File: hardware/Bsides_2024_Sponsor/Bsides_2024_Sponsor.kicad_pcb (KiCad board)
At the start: 2 copper layers, 139.6 x 139.6 mm, 43 parts, among them J2 Battery, J3 Battery, J4 OLED, J5 Add_On, P1 USB_C_Plug_USB2.0, Q1 DMG3415U-7, SW1 ON, SW2 RESET, SW3 BOOT, SW4 RESET, SW6 RESET, U1 ESP32-C6-WROOM-1U-N4, U2 AP2112K-3.3

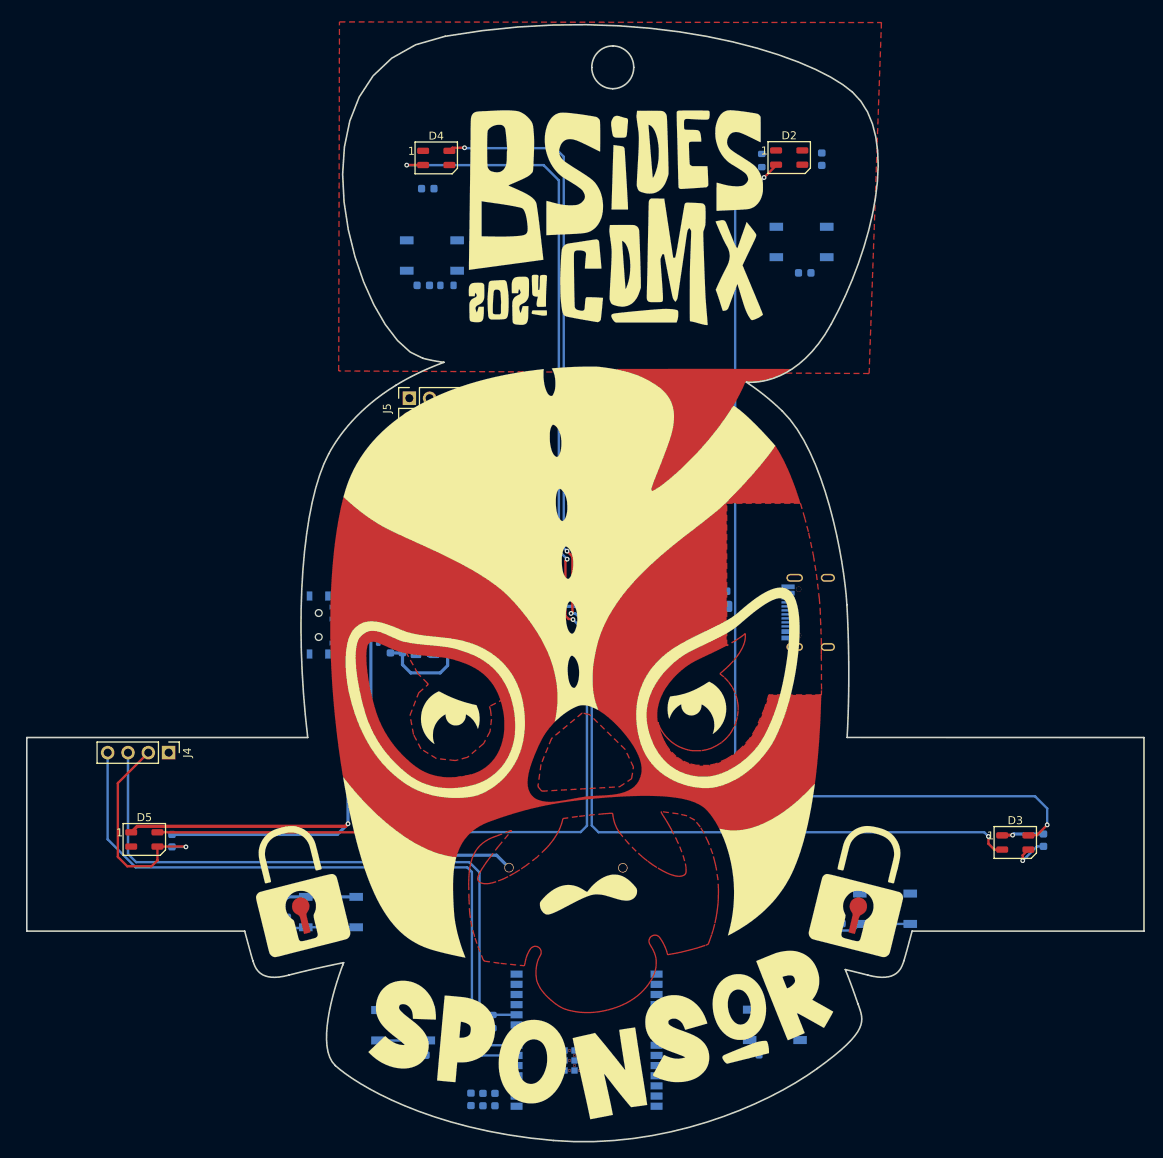
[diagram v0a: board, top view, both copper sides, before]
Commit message: feat(Hw):Update_Route_Sponsor
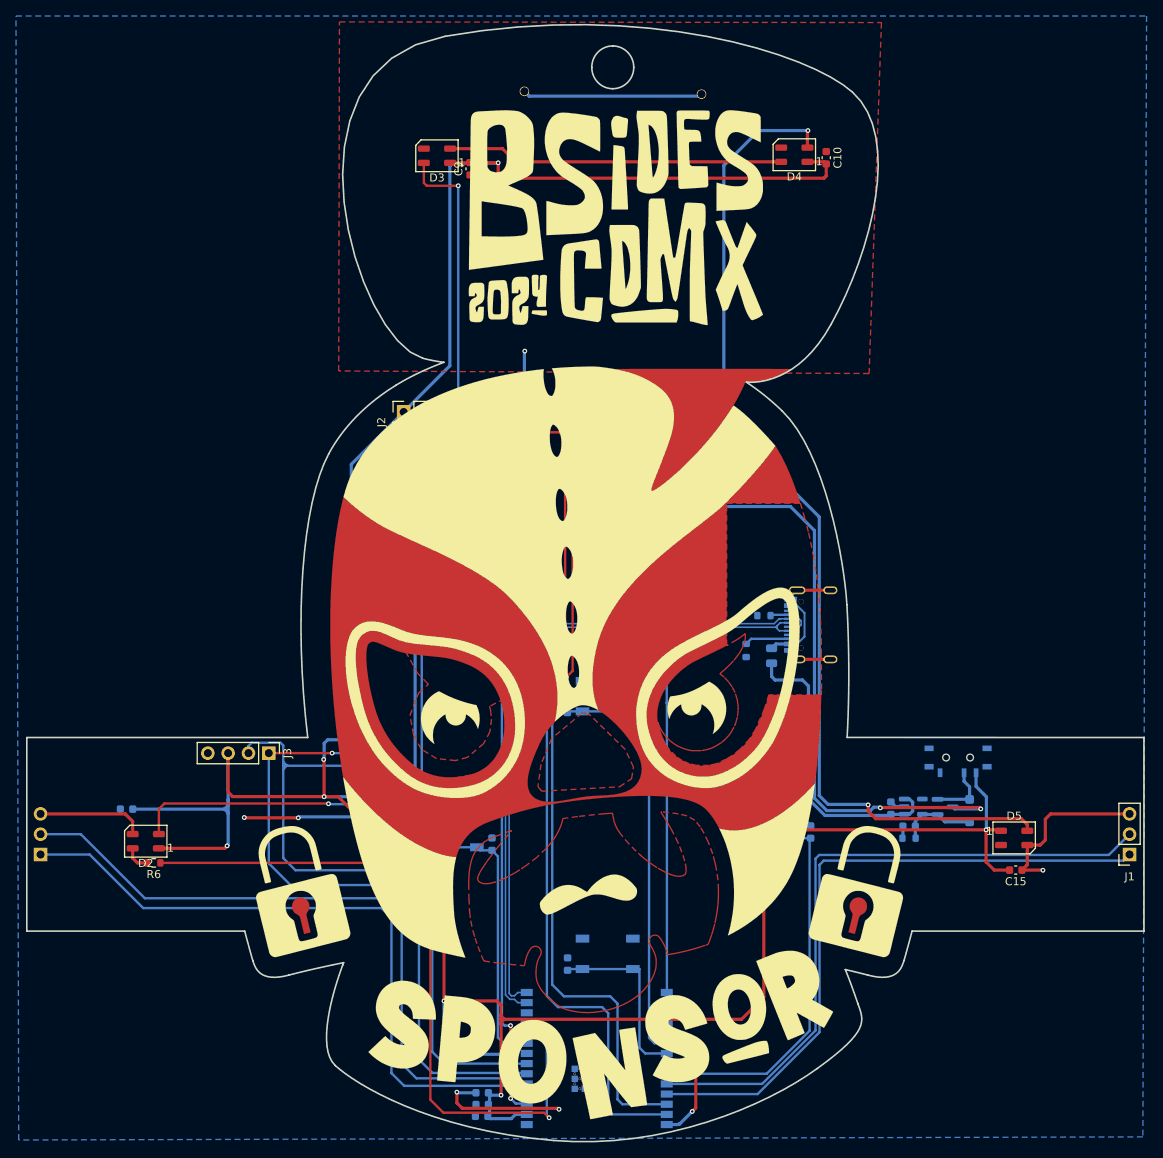
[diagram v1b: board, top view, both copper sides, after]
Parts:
- added J1: Serial_IN, Connector_PinSocket_2.54mm:PinSocket_1x03_P2.54mm_Vertical, F.Cu at (211.0, 126.4)
- added J6: Battery, bsides:BH-AA-A1AJ020, B.Cu at (135.3, 56.8)
- C1: value 10uF -> 1uF
- C10, C9, R6: moved to F.Cu
- C13: value 1uF -> 0.1uF
- C14: value 10uF -> 0.1uF
- C15: value 10uF -> 0.1uF; moved to F.Cu
- C3, C4, C5: value 0.1uF -> 10uF
- J2: value Battery -> Add_On; footprint bsides:BH-AAA-A1aj001 -> Connector_PinSocket_2.54mm:PinSocket_2x03_P2.54mm_Vertical; moved to F.Cu
- J3: value Battery -> OLED; footprint bsides:BH-AAA-A1aj001 -> bsides:Display OLED 128 x32; moved to F.Cu
- J4: value OLED -> Serial_OUT; footprint bsides:Display OLED 128 x32 -> Connector_PinHeader_2.54mm:PinHeader_1x03_P2.54mm_Vertical; moved to B.Cu
- J5: value Add_On -> Battery; footprint Connector_PinSocket_2.54mm:PinSocket_2x03_P2.54mm_Vertical -> bsides:BH-AA-A1AJ020; moved to B.Cu
- U1: value ESP32-C6-WROOM-1U-N4 -> ESP32-C6-WROOM-1-N4
- moved D2 117.3 mm to (88.0, 124.8), turned to 180 degrees
- moved R6 116.1 mm to (89.0, 127.5), turned to 180 degrees
- moved C3 112.9 mm to (130.0, 159.2)
- moved C10 112.5 mm to (173.1, 39.3), turned to -90 degrees
- moved D3 112.2 mm to (124.4, 39.1), turned to 180 degrees
- moved D5 108.7 mm to (196.5, 124.4)
- moved C9 96.5 mm to (128.5, 40.7), turned to 90 degrees
- moved C8 89.8 mm to (85.6, 120.8), turned to 0 degrees
- moved C4 87.7 mm to (181.1, 120.7), turned to 90 degrees
- moved C6 86.5 mm to (123.2, 85.3), turned to -90 degrees
- moved C5 84.1 mm to (183.4, 122.9), turned to 180 degrees
- moved SW1 81.6 mm to (189.5, 114.3), turned to 0 degrees
- moved C12 79.8 mm to (171.1, 123.6), turned to -90 degrees
- moved D1 78.9 mm to (191.0, 121.0), turned to -90 degrees
- moved Q1 75.0 mm to (187.9, 120.5), turned to 0 degrees
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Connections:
- C1 pad 1: VBUS -> /VOUT
- C10 pad 2: /GPIO15 -> /VOUT
- C11 pad 2: /GPIO23 -> /GPIO1
- C12 pad 2: /VOUT -> /GPIO15
- C13 pad 1: /VOUT -> GND
- C13 pad 2: GND -> /GPIO22
- C14 pad 1: /VOUT -> GND
- C14 pad 2: GND -> /GPIO23
- C15 pad 1: /VOUT -> GND
- C15 pad 2: GND -> /VOUT
- C2 pad 1: Net-(D1-A) -> /VOUT
- C3 pad 1: GND -> /VOUT
- C3 pad 2: /BOOT -> GND
- C4 pad 1: GND -> VBUS
- C4 pad 2: /EN -> GND
- C5 pad 1: GND -> Net-(D1-A)
- C5 pad 2: /VOUT -> GND
- C6 pad 2: /VOUT -> /BOOT
- C7 pad 2: /VOUT -> /EN
- C8 pad 2: /GPIO1 -> /VOUT
- C9 pad 2: /GPIO22 -> /VOUT
- J2 pad 1: Net-(J2-Pin_1) -> /VOUT
- J2 pad 2: +BATT -> GND
- J3 pad 1: GND -> /SDA
- J3 pad 2: Net-(J2-Pin_1) -> /SCL
- J4 pad 1: /VOUT -> /GPIO4
- J4 pad 2: GND -> /GPIO5
- J4 pad 3: /SCL -> GND
- J5 pad 1: /VOUT -> Net-(J5-Pin_1)
- J5 pad 2: GND -> +BATT
- R1 pad 1: /PIN -> Net-(U1-IO8)
- SW1 pad 2: /VOUT -> Net-(D1-K)
- SW1 pad 3: Net-(D1-K) -> /VOUT
- SW5 pad 2: /GPIO22 -> /GPIO15
- SW6 pad 2: /GPIO15 -> /GPIO22
- U1 pad 10: /PIN -> Net-(U1-IO8)
- U1 pad 11: unconnected-(U1-IO10-Pad11) -> /PIN
- U1 pad 24: /RX -> /GPIO17
- U1 pad 25: /TX -> /GPIO16
- U1 pad 26: unconnected-(U1-IO3-Pad26) -> /GPIO3
- U1 pad 27: unconnected-(U1-IO2-Pad27) -> /GPIO2
- U1 pad 4: unconnected-(U1-IO4-Pad4) -> /GPIO4
- U1 pad 5: unconnected-(U1-IO5-Pad5) -> /GPIO5
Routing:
- net /VOUT: track 82.4 -> 402.0 mm, vias 2 -> 7
- net /GPIO3: track 0.00 -> 115.6 mm, vias 0 -> 1
- net /GPIO2: track 0.00 -> 114.4 mm, vias 0 -> 1
- net Net-(D3-DOUT): track 153.5 -> 42.1 mm, vias 4 -> 0
- net /BOOT: track 0.00 -> 95.5 mm, vias 0 -> 2
- net GND: track 56.8 -> 146.8 mm, vias 2 -> 10
- net /PIN: track 2.97 -> 90.1 mm, vias 0 -> 1
- net /D-: track 0.00 -> 86.6 mm
- net /GPIO5: track 0.00 -> 84.7 mm
- net /GPIO4: track 0.00 -> 84.5 mm
- net /D+: track 0.00 -> 84.2 mm
- net /GPIO17: track 0.00 -> 83.4 mm
- net /GPIO16: track 0.00 -> 82.5 mm
- net /EN: track 0.00 -> 80.9 mm, vias 0 -> 2
- net /GPIO15: track 0.00 -> 53.4 mm
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- added copper zone on B.Cu, net GND
